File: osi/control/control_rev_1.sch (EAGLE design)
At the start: 10 parts, among them J1 1X2-3.5MM, J2 1X2-3.5MM

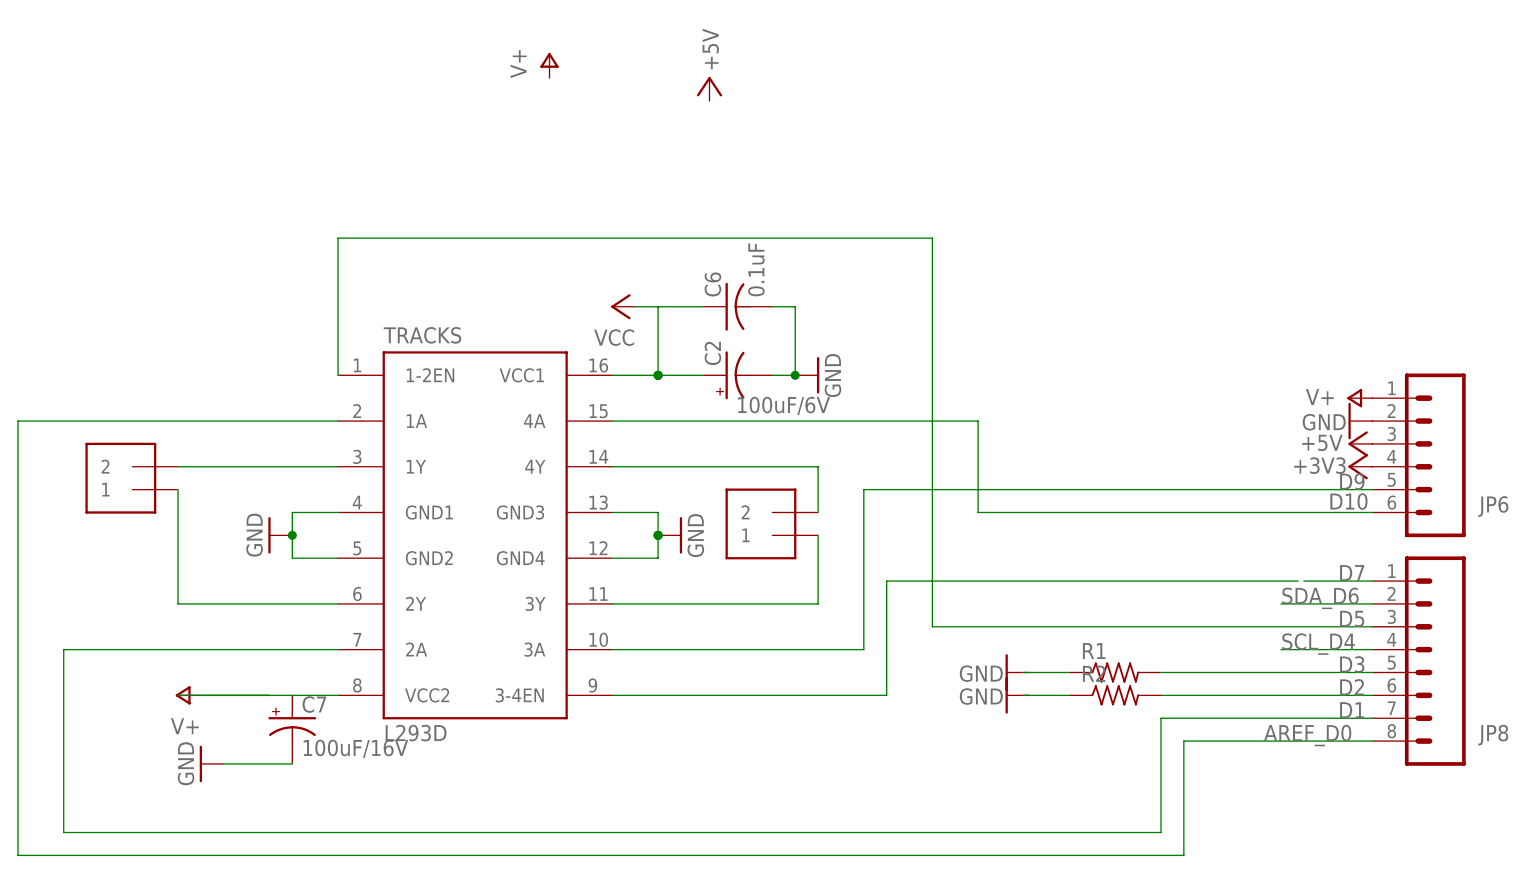
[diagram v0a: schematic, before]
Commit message: update
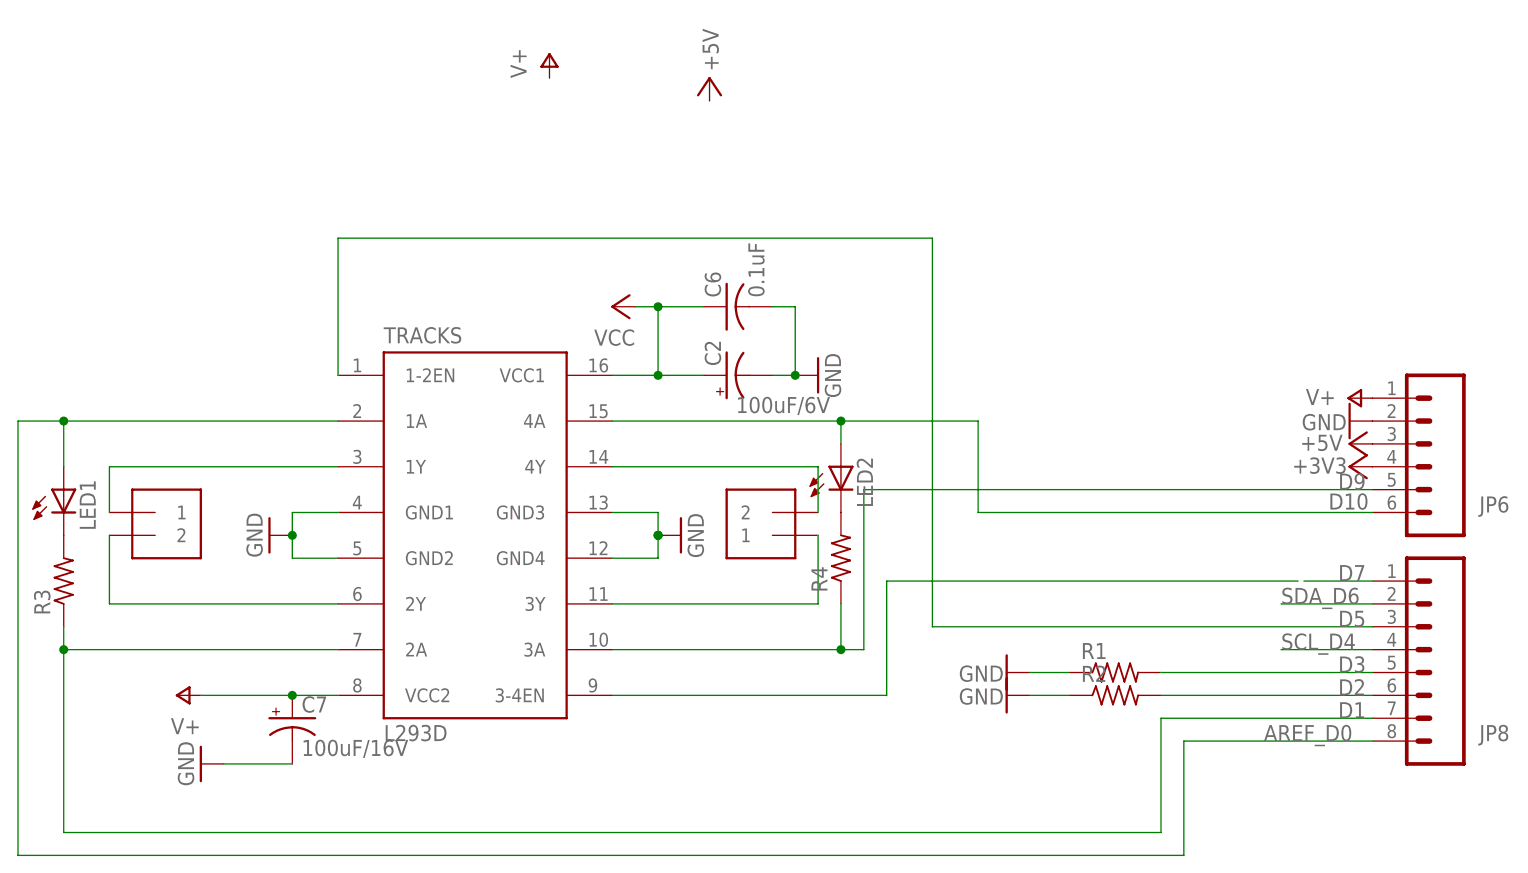
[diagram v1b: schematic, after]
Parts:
- added LED1, LED2: (no value), adafruit:LED3MM
- added R3, R4: (no value), adafruit_mod:R-US_0204/2V
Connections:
- net AREF_D0: now also LED1.A
- net D1: now also R3.1
- net D10: now also LED2.A
- net D9: now also R4.1
- net GND: now also R1.1, R2.1
- net N$1: now also J1.1; no longer J1.2
- net N$3: now also J1.2; no longer J1.1
- net N$6: now also LED1.C, R3.2; no longer R1.1
- net N$7: now also LED2.C, R4.2; no longer R2.1
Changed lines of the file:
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@@
 <setting verticaltext="up"/>
 </settings>
-<grid distance="0.1" unitdist="inch" unit="inch" style="lines" multiple="1" display="no" altdistance="0.001" altunitdist="inch" altunit="inch"/>
+<grid distance="0.1" unitdist="inch" unit="inch" style="lines" multiple="1" display="no" altdistance="0.01" altunitdist="inch" altunit="inch"/>
 <layers>
 <layer number="1" name="Top" color="4" fill="1" visible="no" active="no"/>
@@
 <part name="GND1" library="SparkFun" deviceset="GND" device=""/>
 <part name="GND2" library="SparkFun" deviceset="GND" device=""/>
+<part name="LED1" library="adafruit" deviceset="LED" device="3MM"/>
+<part name="LED2" library="adafruit" deviceset="LED" device="3MM"/>
+<part name="R3" library="adafruit_mod" deviceset="R-US_" device="0204/2V"/>
+<part name="R4" library="adafruit_mod" deviceset="R-US_" device="0204/2V"/>
 </parts>
 <sheets>
@@
 <instance part="C6" gate="G$1" x="119.38" y="106.68" rot="R90"/>
 <instance part="P+10" gate="1" x="58.42" y="63.5" rot="R90"/>
-<instance part="J1" gate="G$1" x="53.34" y="88.9" rot="R180"/>
+<instance part="J1" gate="G$1" x="55.88" y="81.28"/>
 <instance part="J2" gate="G$1" x="124.46" y="83.82" rot="R180"/>
 <instance part="R1" gate="G$1" x="162.56" y="66.04"/>
@@
 <attribute name="VALUE" x="145.161" y="62.484" size="1.778" layer="96"/>
 </instance>
+<instance part="LED1" gate="G$1" x="45.72" y="86.36"/>
+<instance part="LED2" gate="G$1" x="132.08" y="88.9"/>
+<instance part="R3" gate="G$1" x="45.72" y="76.2" rot="R90"/>
+<instance part="R4" gate="G$1" x="132.08" y="78.74" rot="R90"/>
 </instances>
 <busses>
@@
 <junction x="111.76" y="81.28"/>
 </segment>
+<segment>
+<pinref part="R1" gate="G$1" pin="1"/>
+<pinref part="GND1" gate="1" pin="GND"/>
+<wire x1="153.035" y1="66.04" x2="157.48" y2="66.04" width="0.1524" layer="91"/>
+</segment>
+<segment>
+<pinref part="R2" gate="G$1" pin="1"/>
+<pinref part="GND2" gate="1" pin="GND"/>
+<wire x1="153.035" y1="63.5" x2="157.48" y2="63.5" width="0.1524" layer="91"/>
+</segment>
 </net>
 <net name="D3" class="0">
@@
 <wire x1="167.64" y1="48.26" x2="167.64" y2="60.96" width="0.1524" layer="91"/>
 <wire x1="167.64" y1="60.96" x2="191.135" y2="60.96" width="0.1524" layer="91"/>
+<pinref part="R3" gate="G$1" pin="1"/>
+<wire x1="45.72" y1="71.12" x2="45.72" y2="68.58" width="0.1524" layer="91"/>
+<junction x="45.72" y="68.58"/>
 </segment>
 </net>
@@
 <label x="179.07" y="58.42" size="1.778" layer="95"/>
 <pinref part="TRACKS" gate="G$1" pin="1A"/>
-<wire x1="76.2" y1="93.98" x2="40.64" y2="93.98" width="0.1524" layer="91"/>
+<wire x1="76.2" y1="93.98" x2="45.72" y2="93.98" width="0.1524" layer="91"/>
+<wire x1="45.72" y1="93.98" x2="40.64" y2="93.98" width="0.1524" layer="91"/>
 <wire x1="40.64" y1="93.98" x2="40.64" y2="45.72" width="0.1524" layer="91"/>
 <wire x1="40.64" y1="45.72" x2="170.18" y2="45.72" width="0.1524" layer="91"/>
 <wire x1="170.18" y1="45.72" x2="170.18" y2="58.42" width="0.1524" layer="91"/>
 <wire x1="170.18" y1="58.42" x2="191.135" y2="58.42" width="0.1524" layer="91"/>
+<pinref part="LED1" gate="G$1" pin="A"/>
+<wire x1="45.72" y1="88.9" x2="45.72" y2="93.98" width="0.1524" layer="91"/>
+<junction x="45.72" y="93.98"/>
 </segment>
 </net>
@@
 <wire x1="134.62" y1="86.36" x2="134.62" y2="68.58" width="0.1524" layer="91"/>
 <pinref part="TRACKS" gate="G$1" pin="3A"/>
-<wire x1="134.62" y1="68.58" x2="106.68" y2="68.58" width="0.1524" layer="91"/>
+<wire x1="134.62" y1="68.58" x2="132.08" y2="68.58" width="0.1524" layer="91"/>
+<pinref part="R4" gate="G$1" pin="1"/>
+<wire x1="132.08" y1="68.58" x2="106.68" y2="68.58" width="0.1524" layer="91"/>
+<wire x1="132.08" y1="73.66" x2="132.08" y2="68.58" width="0.1524" layer="91"/>
+<junction x="132.08" y="68.58"/>
 </segment>
 </net>
@@
 </segment>
 <segment>
-<wire x1="71.12" y1="63.5" x2="76.2" y2="63.5" width="0.1524" layer="91"/>
 <pinref part="TRACKS" gate="G$1" pin="VCC2"/>
+<pinref part="P+10" gate="1" pin="V+"/>
+<wire x1="76.2" y1="63.5" x2="71.12" y2="63.5" width="0.1524" layer="91"/>
 <pinref part="C7" gate="G$1" pin="+"/>
-<wire x1="71.12" y1="63.5" x2="68.58" y2="63.5" width="0.2032" layer="91"/>
-<pinref part="P+10" gate="1" pin="V+"/>
-<wire x1="68.58" y1="63.5" x2="60.96" y2="63.5" width="0.2032" layer="91"/>
-<wire x1="68.58" y1="63.5" x2="58.42" y2="63.5" width="0.2032" layer="91"/>
-</segment>
-</net>
-<net name="VCC" class="0">
-<segment>
-<wire x1="116.84" y1="99.06" x2="111.76" y2="99.06" width="0.1524" layer="91"/>
-<wire x1="111.76" y1="99.06" x2="106.68" y2="99.06" width="0.1524" layer="91"/>
-<wire x1="116.84" y1="106.68" x2="111.76" y2="106.68" width="0.1524" layer="91"/>
-<wire x1="109.22" y1="106.68" x2="111.76" y2="106.68" width="0.1524" layer="91"/>
-<wire x1="111.76" y1="106.68" x2="111.76" y2="99.06" width="0.1524" layer="91"/>
-<junction x="111.76" y="99.06"/>
-<junction x="111.76" y="99.06"/>
-<pinref part="TRACKS" gate="G$1" pin="VCC1"/>
-<pinref part="C2" gate="G$1" pin="+"/>
-<pinref part="C6" gate="G$1" pin="1"/>
-<pinref part="+5V1" gate="VCC" pin="VCC"/>
-</segment>
-</net>
-<net name="N$1" class="0">
-<segment>
-<pinref part="TRACKS" gate="G$1" pin="1Y"/>
+<wire x1="71.12" y1="63.5" x2="60.96" y2="63.5" width="0.1524" layer="91"/>
+<junction x="71.12" y="63.5"/>
+</segment>
+</net>
+<net name="N$3" class="0">
+<segment>
+<pinref part="TRACKS" gate="G$1" pin="2Y"/>
+<wire x1="76.2" y1="73.66" x2="50.8" y2="73.66" width="0.1524" layer="91"/>
 <pinref part="J1" gate="G$1" pin="2"/>
-<wire x1="58.42" y1="88.9" x2="76.2" y2="88.9" width="0.1524" layer="91"/>
-</segment>
-</net>
-<net name="N$3" class="0">
-<segment>
-<pinref part="TRACKS" gate="G$1" pin="2Y"/>
-<pinref part="J1" gate="G$1" pin="1"/>
-<wire x1="76.2" y1="73.66" x2="58.42" y2="73.66" width="0.1524" layer="91"/>
-<wire x1="58.42" y1="73.66" x2="58.42" y2="86.36" width="0.1524" layer="91"/>
+<wire x1="50.8" y1="73.66" x2="50.8" y2="81.28" width="0.1524" layer="91"/>
 </segment>
 </net>
@@
 <wire x1="147.32" y1="83.82" x2="147.32" y2="93.98" width="0.1524" layer="91"/>
 <pinref part="TRACKS" gate="G$1" pin="4A"/>
-<wire x1="147.32" y1="93.98" x2="106.68" y2="93.98" width="0.1524" layer="91"/>
+<wire x1="147.32" y1="93.98" x2="132.08" y2="93.98" width="0.1524" layer="91"/>
 <pinref part="JP6" gate="G$1" pin="6"/>
 <label x="190.7286" y="85.9282" size="1.778" layer="95" rot="R180"/>
-</segment>
-</net>
-<net name="N$6" class="0">
-<segment>
-<pinref part="R1" gate="G$1" pin="1"/>
-<wire x1="152.4" y1="66.04" x2="157.48" y2="66.04" width="0.1524" layer="91"/>
-</segment>
-</net>
-<net name="N$7" class="0">
-<segment>
-<pinref part="R2" gate="G$1" pin="1"/>
-<wire x1="152.4" y1="63.5" x2="157.48" y2="63.5" width="0.1524" layer="91"/>
+<pinref part="LED2" gate="G$1" pin="A"/>
+<wire x1="132.08" y1="93.98" x2="106.68" y2="93.98" width="0.1524" layer="91"/>
+<wire x1="132.08" y1="91.44" x2="132.08" y2="93.98" width="0.1524" layer="91"/>
+<junction x="132.08" y="93.98"/>
 </segment>
 </net>
@@
 </segment>
 </net>
+<net name="N$1" class="0">
+<segment>
+<pinref part="TRACKS" gate="G$1" pin="1Y"/>
+<wire x1="76.2" y1="88.9" x2="50.8" y2="88.9" width="0.1524" layer="91"/>
+<pinref part="J1" gate="G$1" pin="1"/>
+<wire x1="50.8" y1="88.9" x2="50.8" y2="83.82" width="0.1524" layer="91"/>
+</segment>
+</net>
+<net name="VCC" class="0">
+<segment>
+<pinref part="C6" gate="G$1" pin="1"/>
+<pinref part="+5V1" gate="VCC" pin="VCC"/>
+<wire x1="116.84" y1="106.68" x2="111.76" y2="106.68" width="0.1524" layer="91"/>
+<wire x1="111.76" y1="106.68" x2="109.22" y2="106.68" width="0.1524" layer="91"/>
+<wire x1="116.84" y1="99.06" x2="111.76" y2="99.06" width="0.1524" layer="91"/>
+<pinref part="TRACKS" gate="G$1" pin="VCC1"/>
+<pinref part="C2" gate="G$1" pin="+"/>
+<wire x1="111.76" y1="99.06" x2="106.68" y2="99.06" width="0.1524" layer="91"/>
+<wire x1="111.76" y1="106.68" x2="111.76" y2="99.06" width="0.1524" layer="91"/>
+<junction x="111.76" y="106.68"/>
+<junction x="111.76" y="99.06"/>
+</segment>
+</net>
+<net name="N$6" class="0">
+<segment>
+<pinref part="LED1" gate="G$1" pin="C"/>
+<pinref part="R3" gate="G$1" pin="2"/>
+</segment>
+</net>
+<net name="N$7" class="0">
+<segment>
+<pinref part="LED2" gate="G$1" pin="C"/>
+<pinref part="R4" gate="G$1" pin="2"/>
+</segment>
+</net>
